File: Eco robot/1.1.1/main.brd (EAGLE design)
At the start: 61.5 x 56 mm, 109 parts, among them IC1 REGULATERLM1058, IC2 REGULATERLM1058, Q1 CRYSTALNX5032GA, SW1 SWITCH_4PALPS, SW2 SWITCH_4PALPS, U1 FT232RL, X2 MINI-USB-SHIELD-UX60A-MB-5ST

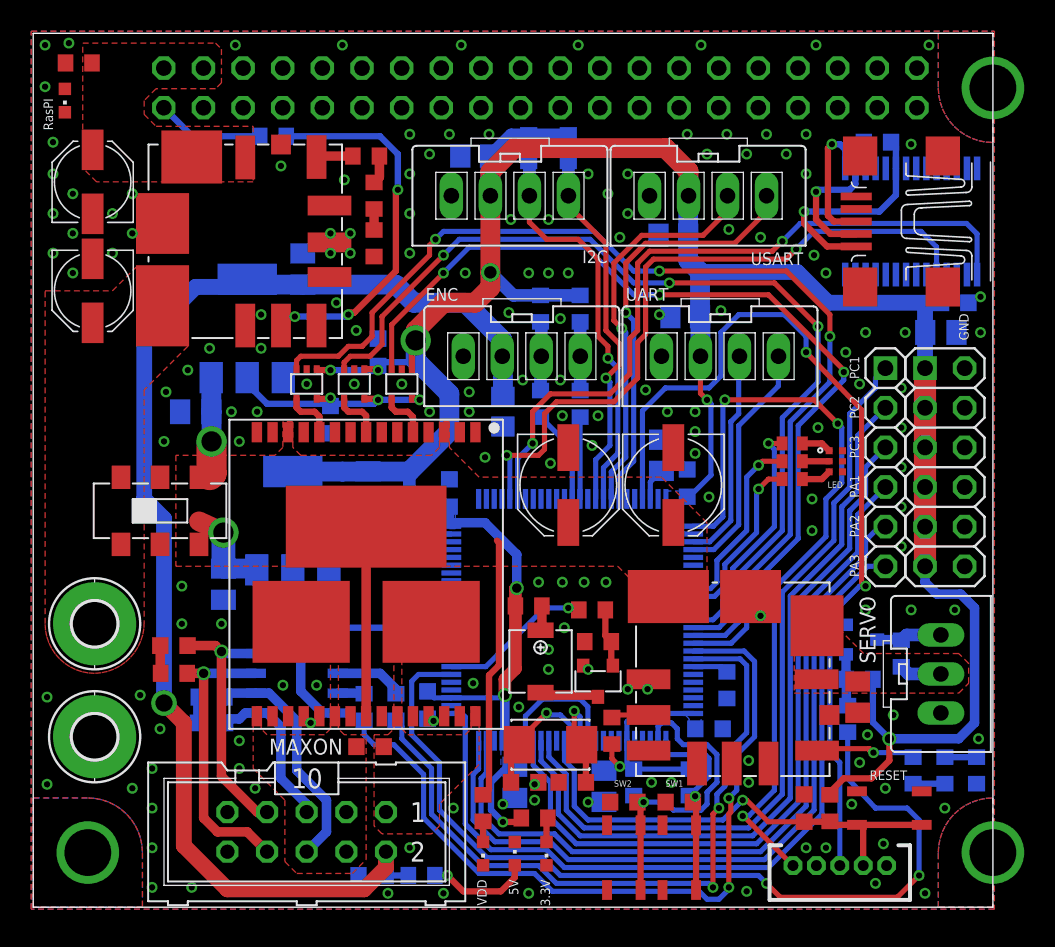
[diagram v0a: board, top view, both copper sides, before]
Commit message: eco new
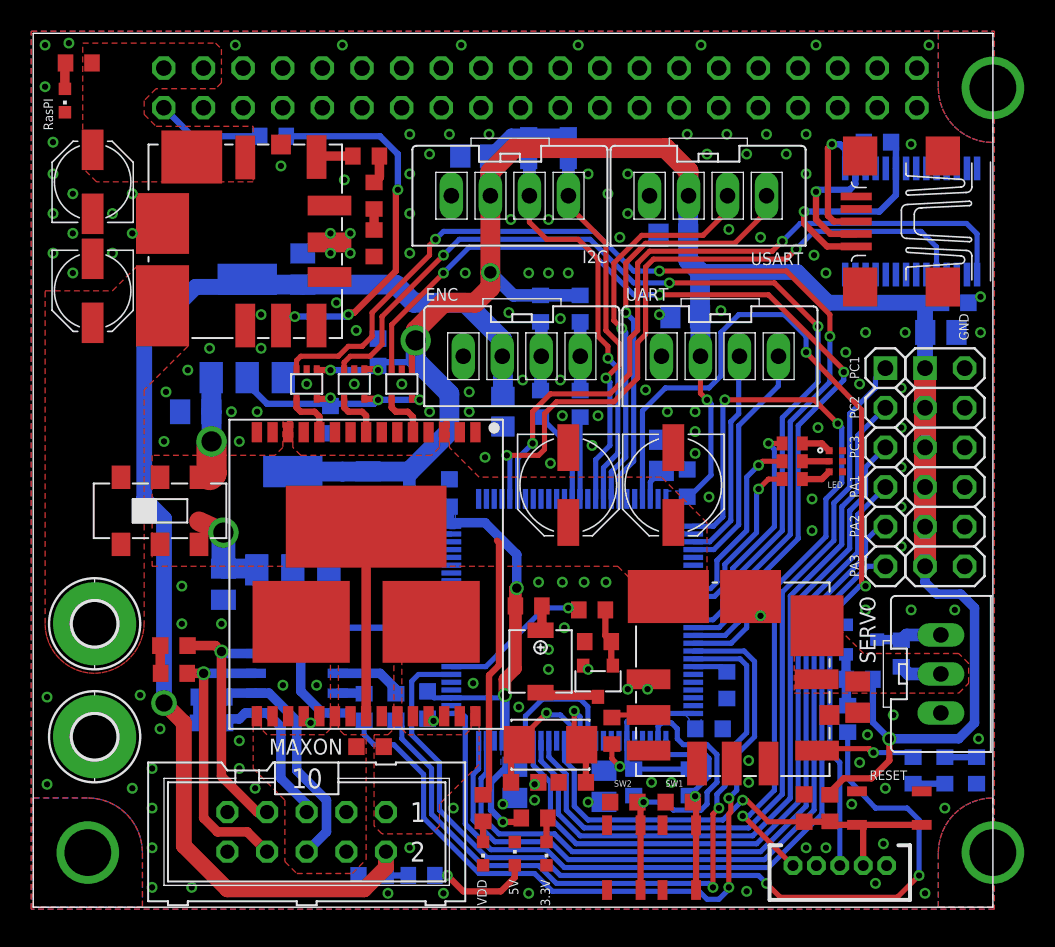
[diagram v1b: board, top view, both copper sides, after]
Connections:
- net VDD: now also U$4.2, U$4.5
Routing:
- net N$9: track 0.00 -> 1.70 mm
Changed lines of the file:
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@@
 <layer number="23" name="tOrigins" color="15" fill="1" visible="yes" active="yes"/>
 <layer number="24" name="bOrigins" color="15" fill="1" visible="yes" active="yes"/>
-<layer number="25" name="tNames" color="7" fill="1" visible="yes" active="yes"/>
-<layer number="26" name="bNames" color="7" fill="1" visible="yes" active="yes"/>
+<layer number="25" name="tNames" color="7" fill="1" visible="no" active="yes"/>
+<layer number="26" name="bNames" color="7" fill="1" visible="no" active="yes"/>
 <layer number="27" name="tValues" color="7" fill="1" visible="no" active="yes"/>
 <layer number="28" name="bValues" color="7" fill="1" visible="no" active="yes"/>
@@
 <text x="1.27" y="49.784" size="0.6096" layer="21" rot="R90">RasPI</text>
 <wire x1="48.133" y1="9.525" x2="48.514" y2="9.525" width="0.254" layer="41"/>
-<wire x1="7.62" y1="21.844" x2="8.636" y2="21.844" width="0.254" layer="41"/>
-<wire x1="7.62" y1="28.956" x2="8.636" y2="28.956" width="0.254" layer="41"/>
 <text x="25.146" y="38.862" size="0.8128" layer="21">ENC</text>
 <text x="35.179" y="41.275" size="0.8128" layer="21">I2C</text>
@@
 <polygon width="0.254" layer="1" isolate="0.254" thermals="no">
 <vertex x="15.494" y="28.956"/>
-<vertex x="9.144" y="28.956"/>
-<vertex x="9.144" y="21.844"/>
+<vertex x="7.62" y="28.956"/>
+<vertex x="7.62" y="21.844"/>
 <vertex x="37.465" y="21.844"/>
 <vertex x="38.481" y="20.828"/>
@@
 <wire x1="11.43" y1="29.845" x2="11.43" y2="27.813" width="1.9304" layer="1"/>
 <wire x1="11.43" y1="27.813" x2="11.303" y2="27.686" width="1.9304" layer="1"/>
+<contactref element="U$4" pad="2"/>
+<contactref element="U$4" pad="5"/>
 </signal>
 <signal name="NRST">
@@
 <contactref element="R11" pad="1"/>
 <contactref element="RASPI" pad="A"/>
-<wire x1="2.032" y1="52.439" x2="2.071" y2="54.102" width="0" layer="19" extent="1-1"/>
+<wire x1="2.071" y1="54.102" x2="2.032" y2="54.102" width="0.6096" layer="1"/>
+<wire x1="2.032" y1="54.102" x2="2.032" y2="52.439" width="0.6096" layer="1"/>
 </signal>
 <signal name="N$15">
